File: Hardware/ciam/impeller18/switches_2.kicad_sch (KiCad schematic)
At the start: 86 parts, among them J11 430451000, J12 430450600, J13 430450400, J14 430450600, J28 430450800, Q23 BSS138, Q24 BSS138, Q25 BSS138, Q26 BSS138, Q27 BSS138, Q28 BSS138, Q29 BSS138, Q30 BSS138, Q31 BSS138, Q32 BSS138, Q33 BSS138, Q34 BSS138, Q35 BSS138, U27 TLP291-4, U28 TLP291-4, U29 B0505MT-1WR4, U30 TLP291, U31 TLP291, U32 TLP291, U33 TLP291, U34 TLP291

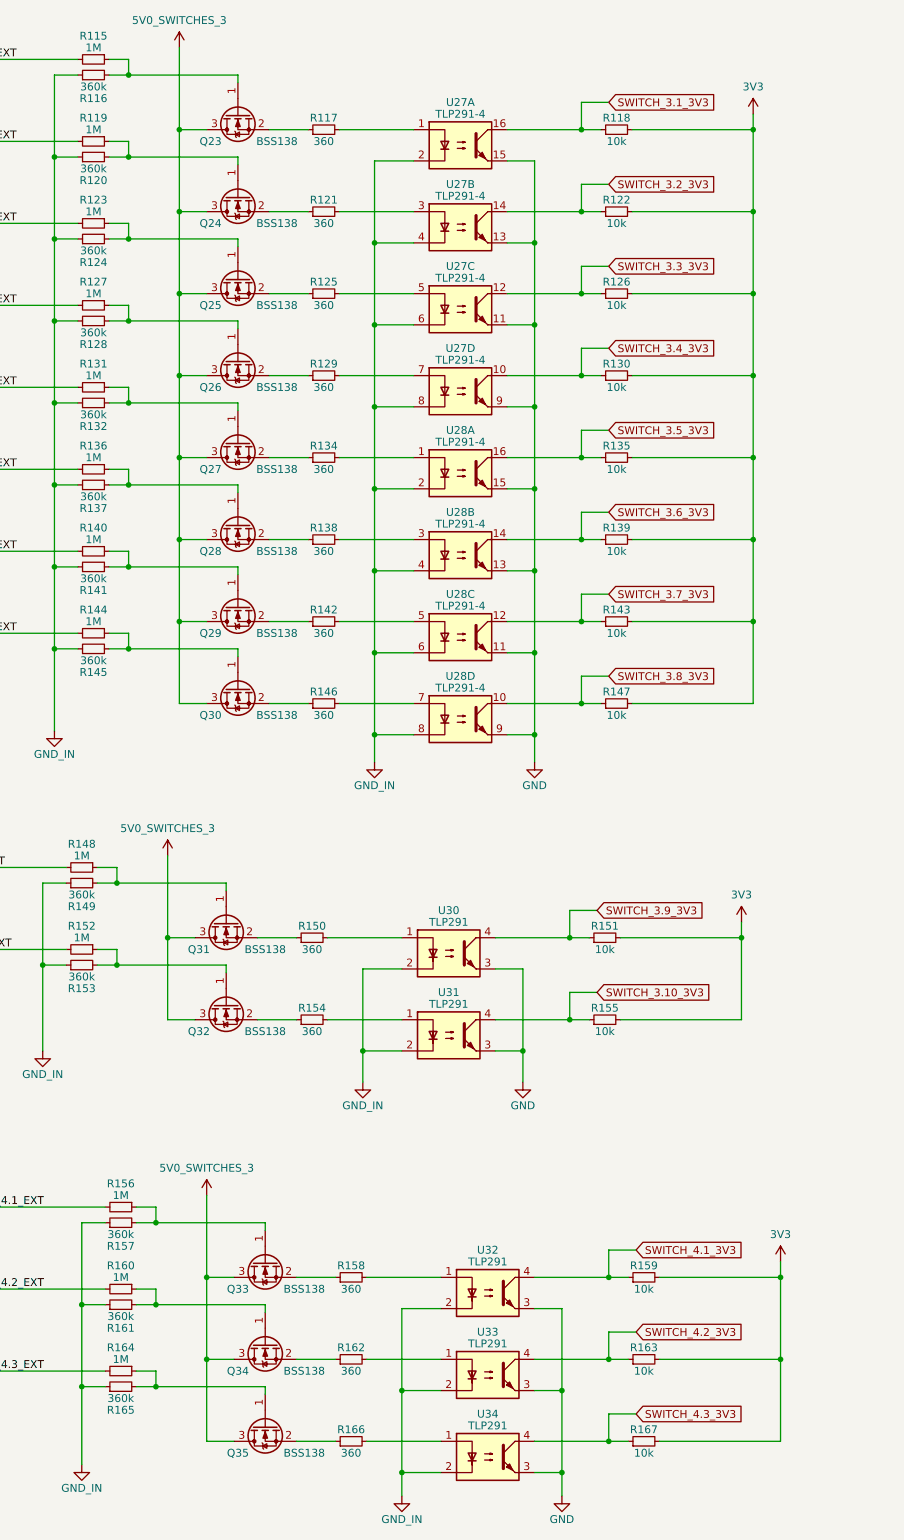
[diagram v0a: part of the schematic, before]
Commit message: fixed switches
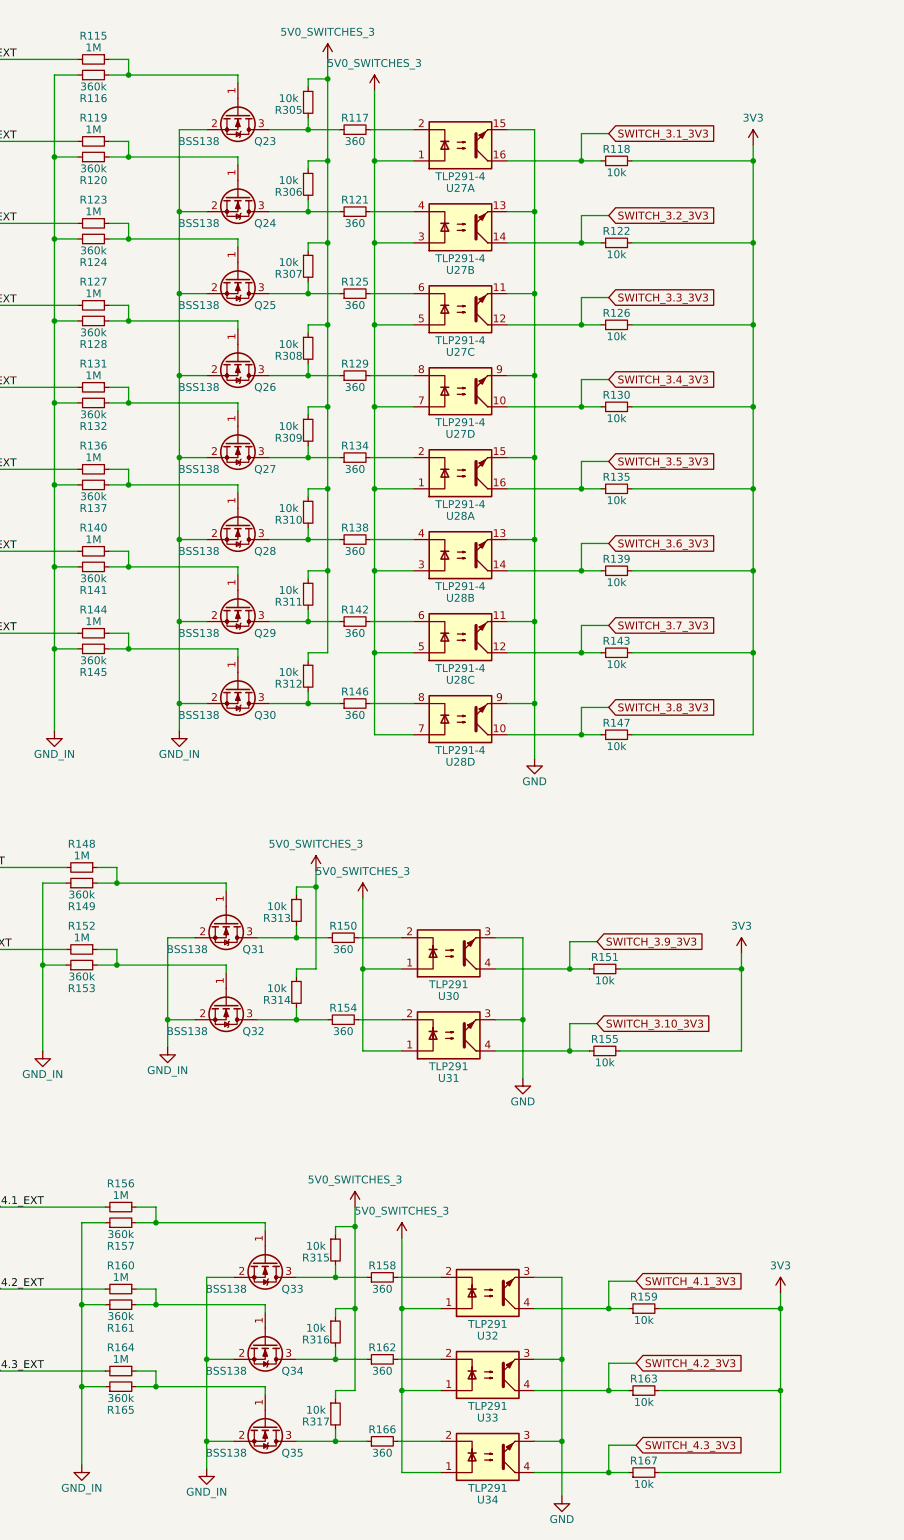
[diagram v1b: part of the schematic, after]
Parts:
- added R305, R306, R307, R308, R309, R310, R311, R312, R313, R314, R315, R316, R317: 10k, Resistor_SMD:R_0603_1608Metric, symbol Device:R_Small
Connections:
- net 5V0_SWITCHES_3: now also U27.1, U27.3, U27.5, U27.7, U28.1, U28.3, U28.5, U28.7, U30.1, U31.1, U32.1, U33.1, U34.1, R305.1, R306.1, R307.1, R308.1, R309.1, R310.1, R311.1, R312.1, R313.1, R314.1, R315.1, R316.1, R317.1; no longer Q23.3 (D), Q24.3 (D), Q25.3 (D), Q26.3 (D), Q27.3 (D), Q28.3 (D), Q29.3 (D), Q30.3 (D), Q31.3 (D), Q32.3 (D), Q33.3 (D), Q34.3 (D), Q35.3 (D)
- net GND_IN: now also Q23.2 (S), Q24.2 (S), Q25.2 (S), Q26.2 (S), Q27.2 (S), Q28.2 (S), Q29.2 (S), Q30.2 (S), Q31.2 (S), Q32.2 (S), Q33.2 (S), Q34.2 (S), Q35.2 (S); no longer U27.2, U27.4, U27.6, U27.8, U28.2, U28.4, U28.6, U28.8, U30.2, U31.2, U32.2, U33.2, U34.2
- net at R158.1: now also Q33.3 (D), R315.2; no longer Q33.2 (S)
- net at R158.2: now also U32.2; no longer U32.1
- net at R146.1: now also Q30.3 (D), R312.2; no longer Q30.2 (S)
- net at R146.2: now also U28.8; no longer U28.7
- net at R117.2: now also U27.2; no longer U27.1
- net at R150.1: now also Q31.3 (D), R313.2; no longer Q31.2 (S)
- net at R150.2: now also U30.2; no longer U30.1
- net at R125.1: now also Q25.3 (D), R307.2; no longer Q25.2 (S)
- net at R142.1: now also Q29.3 (D), R311.2; no longer Q29.2 (S)
- net at R166.2: now also U34.2; no longer U34.1
- net at R154.1: now also Q32.3 (D), R314.2; no longer Q32.2 (S)
- net at R154.2: now also U31.2; no longer U31.1
- net at R121.2: now also U27.4; no longer U27.3
- net at R142.2: now also U28.6; no longer U28.5
- net at R134.1: now also Q27.3 (D), R309.2; no longer Q27.2 (S)
- net at R166.1: now also Q35.3 (D), R317.2; no longer Q35.2 (S)
- net at R162.2: now also U33.2; no longer U33.1
- net at R129.1: now also Q26.3 (D), R308.2; no longer Q26.2 (S)
- net at R138.1: now also Q28.3 (D), R310.2; no longer Q28.2 (S)
- net at R138.2: now also U28.4; no longer U28.3
- net at R121.1: now also Q24.3 (D), R306.2; no longer Q24.2 (S)
- net at R117.1: now also Q23.3 (D), R305.2; no longer Q23.2 (S)
- net at R129.2: now also U27.8; no longer U27.7
- net at R125.2: now also U27.6; no longer U27.5
- net at R162.1: now also Q34.3 (D), R316.2; no longer Q34.2 (S)
- net at R134.2: now also U28.2; no longer U28.1
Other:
- moved on the sheet: Q23, Q24, Q25, Q26, Q27, Q28, Q29, Q30, Q31, Q32, Q33, Q34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

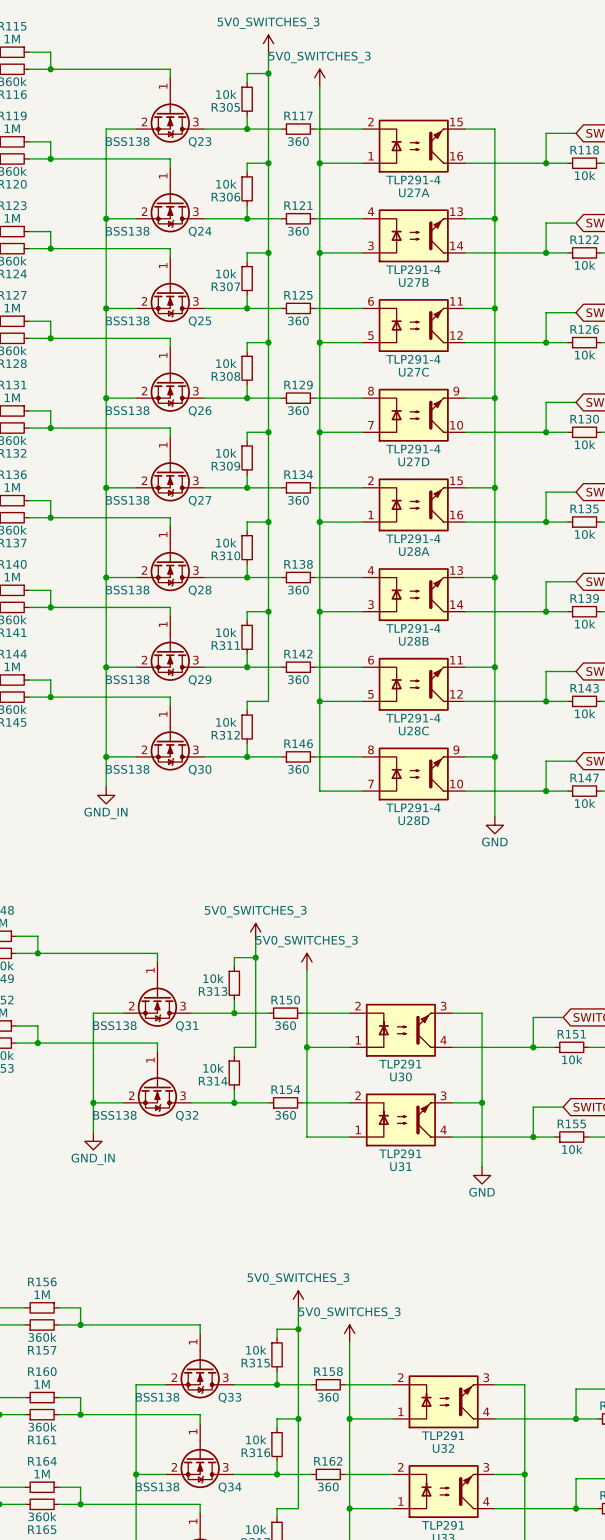
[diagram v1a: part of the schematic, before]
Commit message: Updated packeges
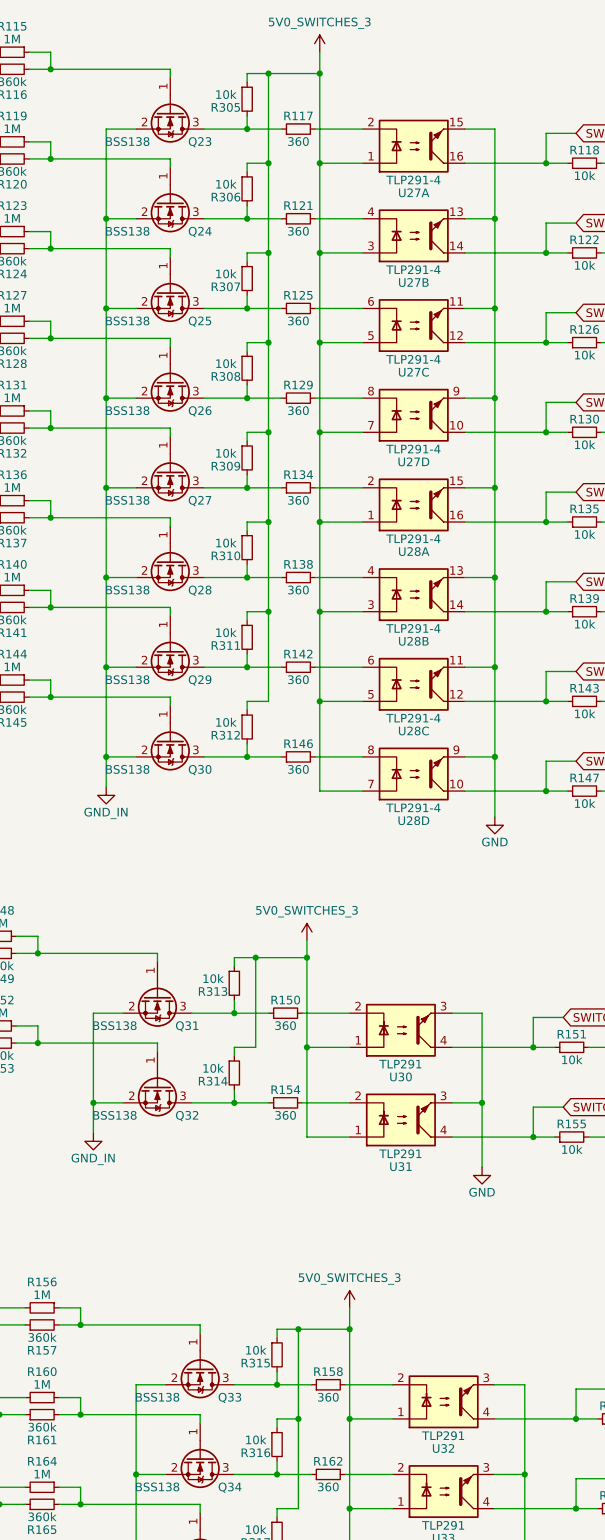
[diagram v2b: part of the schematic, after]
